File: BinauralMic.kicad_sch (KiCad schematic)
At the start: 28 parts, among them IC1 PCM2903CDBR, J1 156-4218-E, J2 USB_C_Receptacle_USB2.0_16P, SW1 SW_Push, SW2 SW_Push, SW3 SW_Push, U1 74LVC1G08, U2 MIC5504-3.3YM5, X1 ECS-120-8-36-CKM-TR3

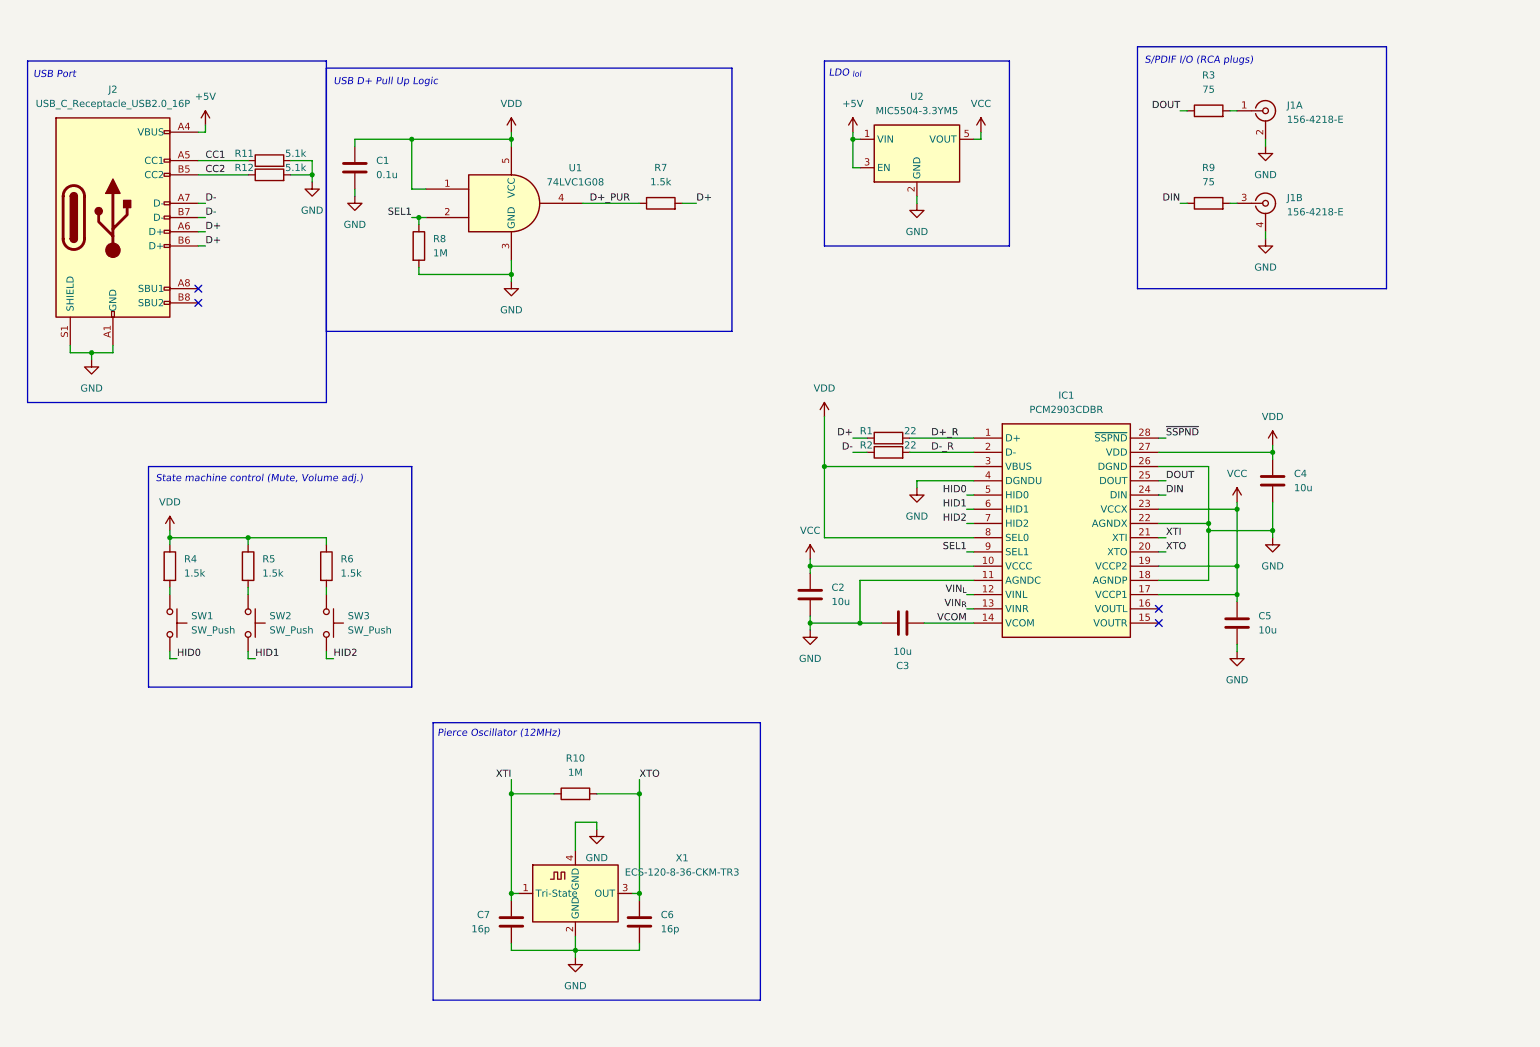
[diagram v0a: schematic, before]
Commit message: Organization
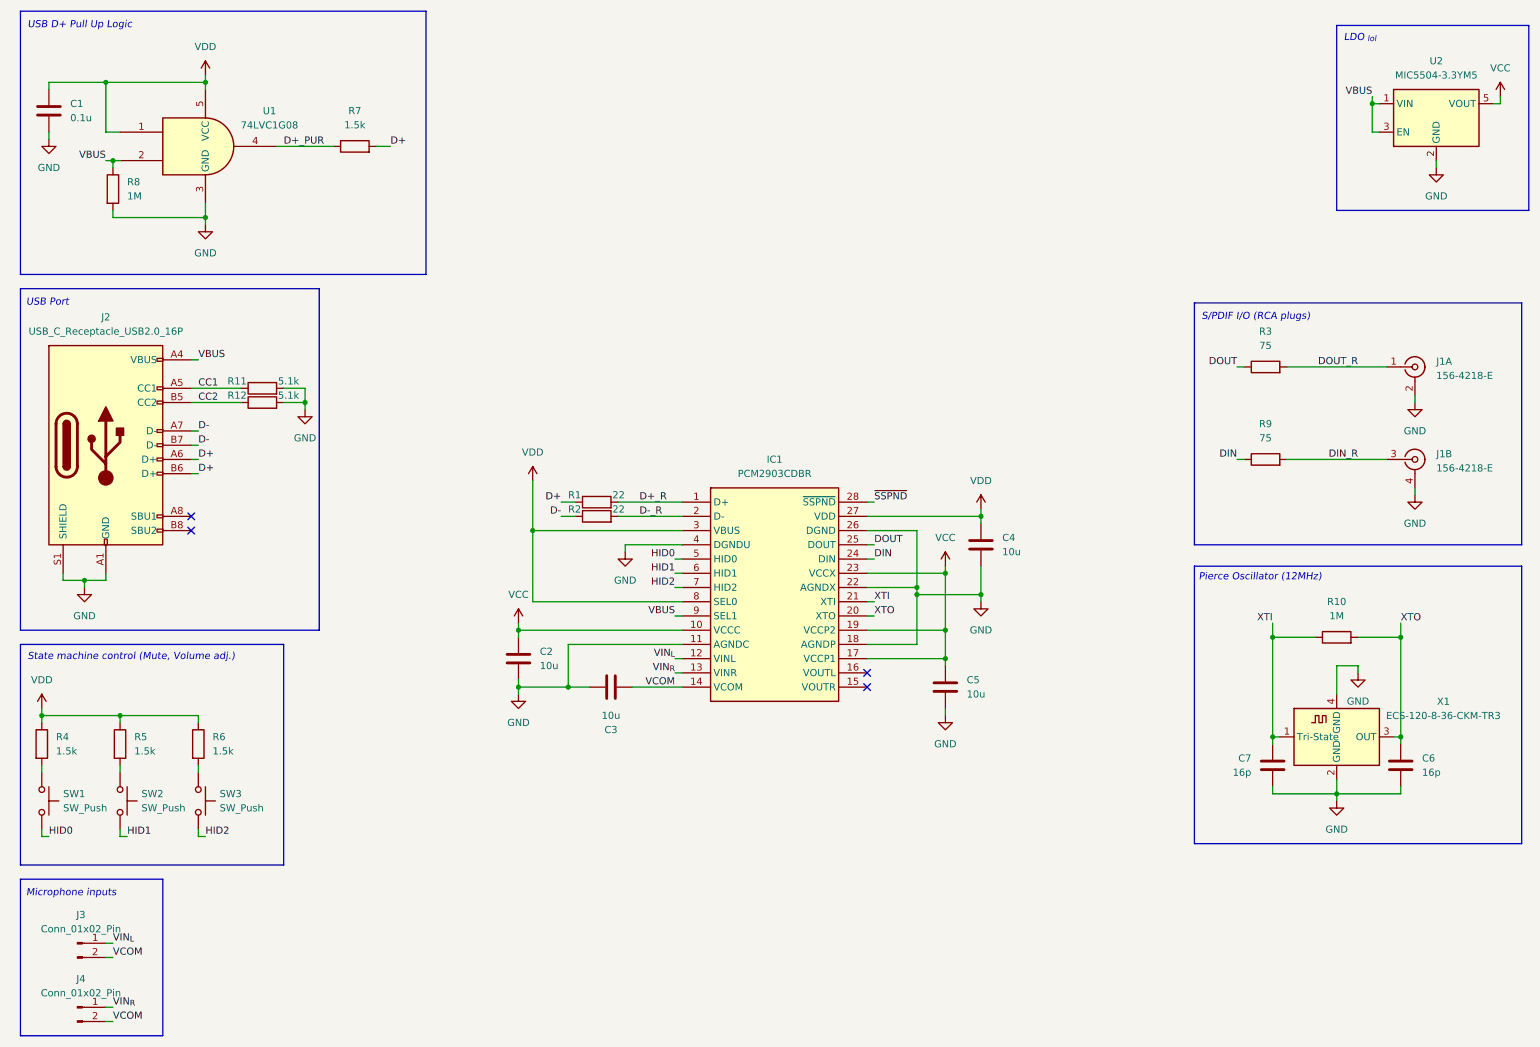
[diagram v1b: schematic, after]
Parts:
- added J3, J4: Conn_01x02_Pin, Connector_PinHeader_2.00mm:PinHeader_1x02_P2.00mm_Vertical, symbol Connector:Conn_01x02_Pin
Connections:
- net SEL1 is gone; now on net VBUS: IC1.9 (SEL1), R8.1, U1.2
- net VCOM: now also J3.2 (Pin_2), J4.2 (Pin_2)
- net VIN_{L}: now also J3.1 (Pin_1)
- net VIN_{R}: now also J4.1 (Pin_1)
- net DOUT_R: now reaches J1.1 (In1), R3.2
- net DIN_R: now reaches J1.3 (In2), R9.2
- net +5V renamed VBUS
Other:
- note added: "Microphone inputs"
- moved on the sheet: C1, C2, C3, C4, C5, C6, C7, IC1, J1A, J1B, J2, R1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
